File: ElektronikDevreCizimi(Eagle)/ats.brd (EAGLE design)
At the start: 90.5 x 74.9 mm, 24 parts, among them IC1 7812TV, IC2 7805TV, Q1 Clock, T1 2N2222, T2 2N2222, U1 ATMEGA328P-PU

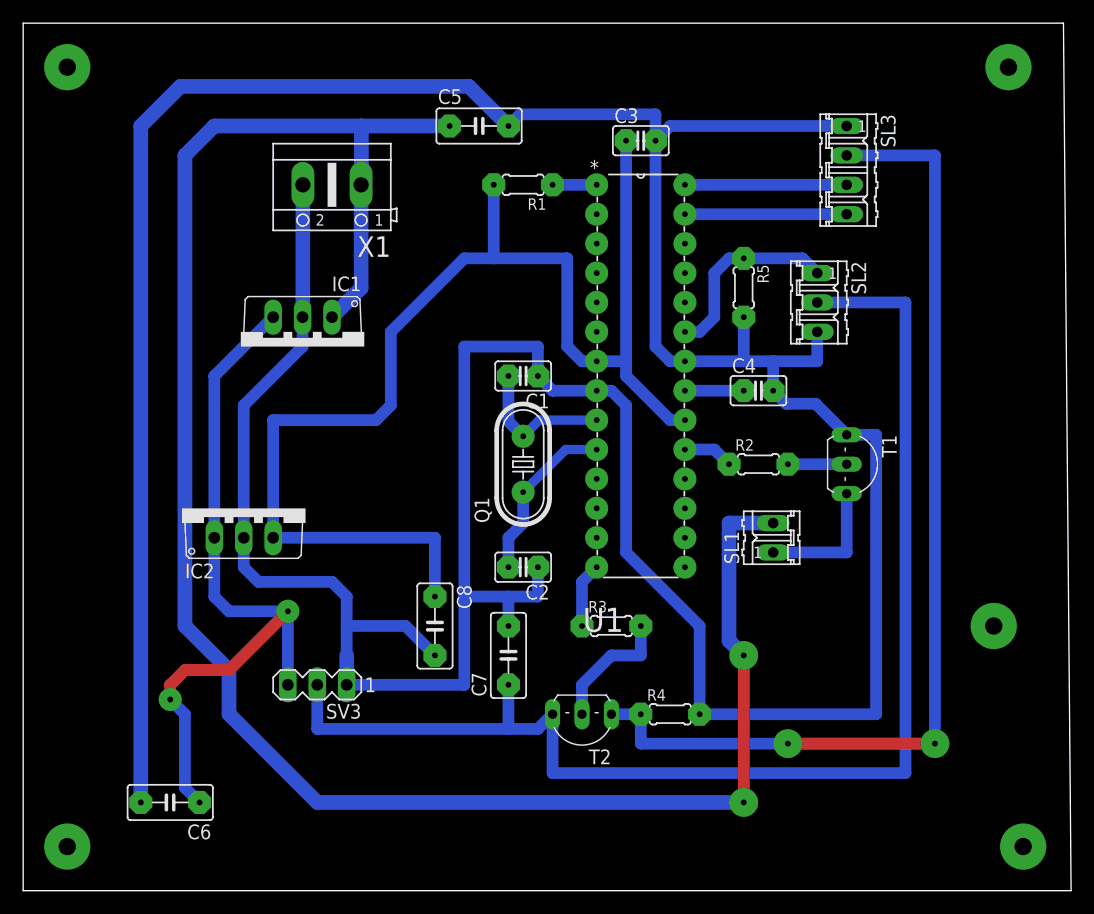
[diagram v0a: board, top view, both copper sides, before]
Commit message: UpdatedAts
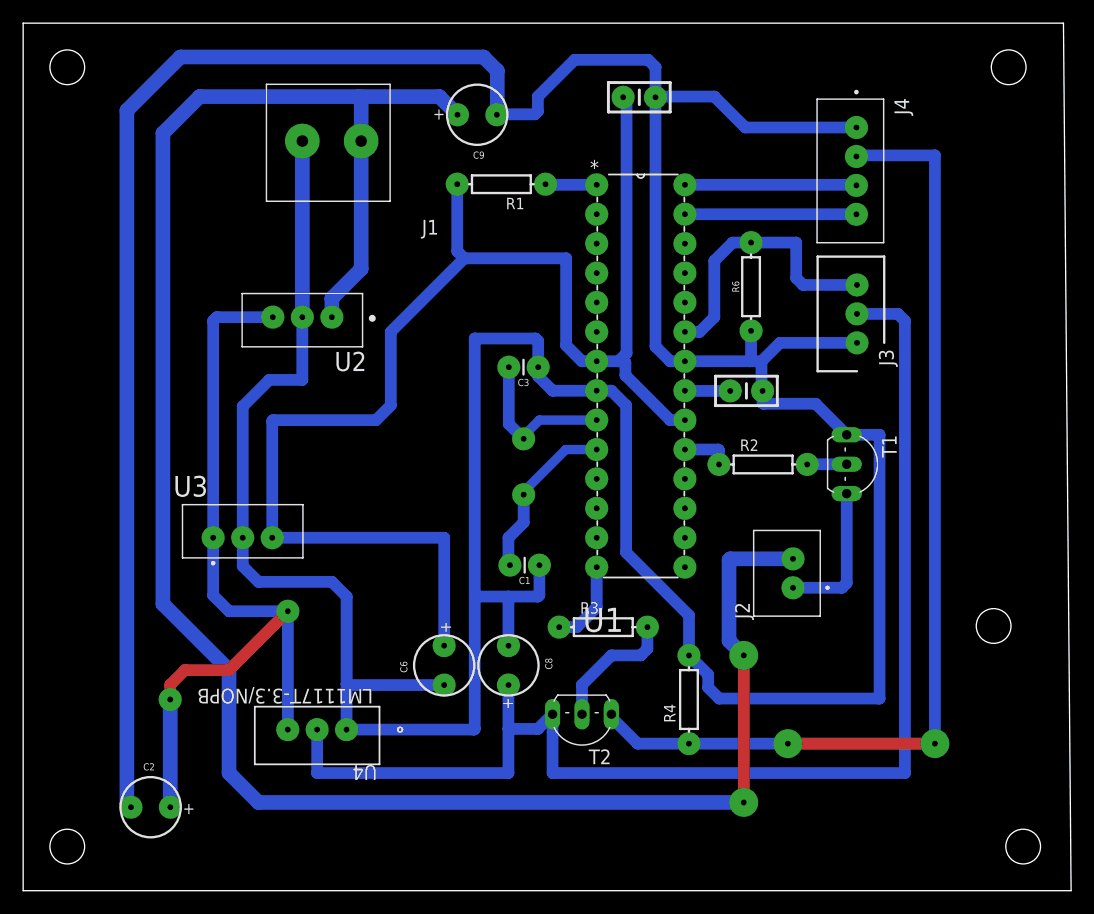
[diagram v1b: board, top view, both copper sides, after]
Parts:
- removed C4: 104, ats_lbr:C025-025X050
- removed IC1: 7812TV, ats_lbr:TO220V
- removed IC2: 7805TV, ats_lbr:TO220V
- removed R5: 10k, ats_lbr:0204/5
- removed SL1: Bzr, con-amp-quick:02P
- removed SL2: Sensor, con-amp-quick:03P
- removed SL3: MainConnect, con-amp-quick:04P
- removed SV3: 3.3VREG, con-lstb:MA03-1
- removed X1: (no value), con-ptr500:AK500/2
- added C9: 0.33 µF, Wurth_Capacitors_WCAP-ATG5-01uf-033uf:WCAP-ATG5_5X11(DXL)
- added J1: 691216510002, 691216510002:691216510002
- added J2: B2B-XH-A(LF)(SN), B2B-XH-A_LF__SN_:JST_B2B-XH-A(LF)(SN)
- added J3: B3B-XH-A_LF__SN_, B3B-XH-A_LF__SN_:SHDR3W64P0X250_1X3_990X575X700
- added J4: B4B-XH-A(LF)(SN), B4B-XH-A_LF__SN_:JST_B4B-XH-A(LF)(SN)
- added R6: 10k, SparkFun-Resistors-10k:AXIAL-0.3
- added U2: L7812CV, L7812CV:TO-220-3
- added U3: L7805CV, L7805CV:TO255P1040X460X1968-3
- added U4: LM1117T-3.3/NOPB, LM1117T:T03B_TEX
- C1: value 22 -> 22pF; device ats_lbr:C025-025X050 -> SparkFun-Capacitors-01uf:CAP-PTH-2.54
- C2: value 22 -> 0.1 µF; device ats_lbr:C025-025X050 -> Wurth_Capacitors_WCAP-ATG5-01uf-033uf:WCAP-ATG5_5X11(DXL)
- C3: value 104 -> 22pF; device ats_lbr:C025-025X050 -> SparkFun-Capacitors-01uf:CAP-PTH-2.54
- C5: value 0.33uf -> 0.1uF; device manken_lbr:C050-030X075 -> SparkFun-Capacitors-01uf:CAP-PTH-SMALL-KIT
- C6: value 0.1uf -> 0.1 µF; device manken_lbr:C050-030X075 -> Wurth_Capacitors_WCAP-ATG5-01uf-033uf:WCAP-ATG5_5X11(DXL)
- C7: value 10uf -> 0.1uF; device manken_lbr:C050-030X075 -> SparkFun-Capacitors-01uf:CAP-PTH-SMALL-KIT
- C8: value 0.1uf -> 10 µF; device manken_lbr:C050-030X075 -> Wurth_Capacitors_WCAP-ATG5-01uf-033uf:WCAP-ATG5_5X11(DXL)
- Q1: device ats_lbr:HC49U-V -> adafruitHC-49S(Buyuk):HC49/S
- R1, R4: device ats_lbr:0204/5 -> SparkFun-Resistors-10k:AXIAL-0.3
- R2, R3: device ats_lbr:0204/5 -> SparkFun-Resistors-1k:AXIAL-0.3
- moved C2 38.3 mm to (7.20, 16.1), turned to 0 degrees
- moved C7 30.7 mm to (58.6, 52.0), turned to 0 degrees
- moved C6 26.5 mm to (32.5, 28.4), turned to 90 degrees
- moved C3 22.0 mm to (39.4, 54.1), turned to 180 degrees
- moved C1 16.3 mm to (39.5, 37.0)
- moved C5 14.1 mm to (49.4, 77.4)
- moved C8 7.20 mm to (38.1, 28.4)
- moved R4 2.06 mm to (53.7, 25.4), turned to 90 degrees
- moved R1 1.88 mm to (37.5, 69.9)
- moved R3 0.71 mm to (46.3, 31.6)
- moved R2 0.40 mm to (60.1, 45.7)
- moved Q1 0.22 mm to (39.4, 45.5), flipped to the bottom
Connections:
- net 12V: now also C2.1, U2.3, U3.1, U4.3; no longer C6.1, IC1.3, IC2.1, SV3.3
- net 24V: now also C9.1, J1.1, J2.2, U2.1; no longer C5.1, IC1.1, SL1.2, X1.1
- net 3.3V: now also C8.1, J3.2, U4.2; no longer C7.1, SL2.2, SV3.2
- net 5V: now also C5.1, C6.1, R1.P$2, U3.3; no longer C3.1, C8.1, IC2.3, R1.2
- net A0: now also J3.3, R6.P$2; no longer R5.1, SL2.1
- net A4: now also J4.4; no longer SL3.4
- net A5: now also J4.3; no longer SL3.3
- net BZR: now also R2.P$1; no longer R2.1
- net GND: now also C2.2, C3.1, C9.2, J1.2, J3.1, J4.1, R4.P$2, R6.P$1, U2.2, U3.2, U4.1; no longer C2.1, C3.2, C4.2, IC1.2, IC2.2, R4.2, R5.2, SL2.3, SL3.1, SV3.1, X1.2
- net N$1: now also R1.P$1; no longer R1.1
- net N$2: now also J2.1; no longer SL1.1
- net N$3: now also R2.P$2; no longer R2.2
- net N$4: now also C3.2; no longer C1.2
- net N$5: now also C1.2; no longer C2.2
- net N$6: now also C7.1; no longer C4.1
- net N$7: now also R3.P$2; no longer R3.2
- net TTK: now also R3.P$1; no longer R3.1
- net TTKMAIN: now also J4.2, R4.P$1; no longer R4.1, SL3.2
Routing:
- net GND: track 375.5 -> 404.6 mm
- net 24V: track 167.4 -> 177.7 mm
- net 5V: track 110.7 -> 120.1 mm
- net A0: track 16.8 -> 24.2 mm
- net 12V: track 63.5 -> 69.6 mm
- net TTKMAIN: track 88.9 -> 86.8 mm
- net TTK: track 5.61 -> 7.41 mm
- net N$3: track 5.08 -> 3.42 mm
- net N$4: track 12.7 -> 13.8 mm
- net N$6: track 5.08 -> 3.92 mm
- net 3.3V: track 112.3 -> 111.1 mm
- net N$2: track 11.4 -> 12.5 mm
- net A5: track 14.0 -> 14.8 mm
- net A4: track 14.0 -> 14.8 mm
- net N$1: track 3.81 -> 4.44 mm
